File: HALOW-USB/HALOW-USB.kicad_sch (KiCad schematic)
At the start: 12 parts, among them U1 TLV75533PDBVR, U2 GT-USB-7010ASV

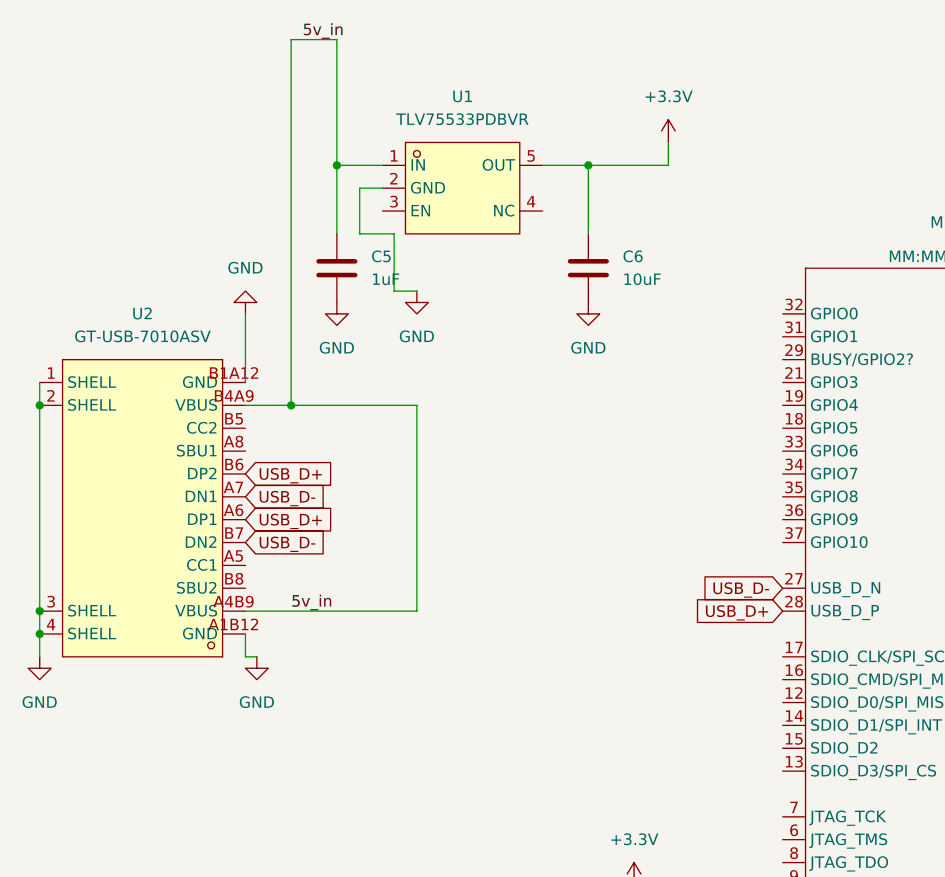
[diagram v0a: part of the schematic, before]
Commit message: trace work
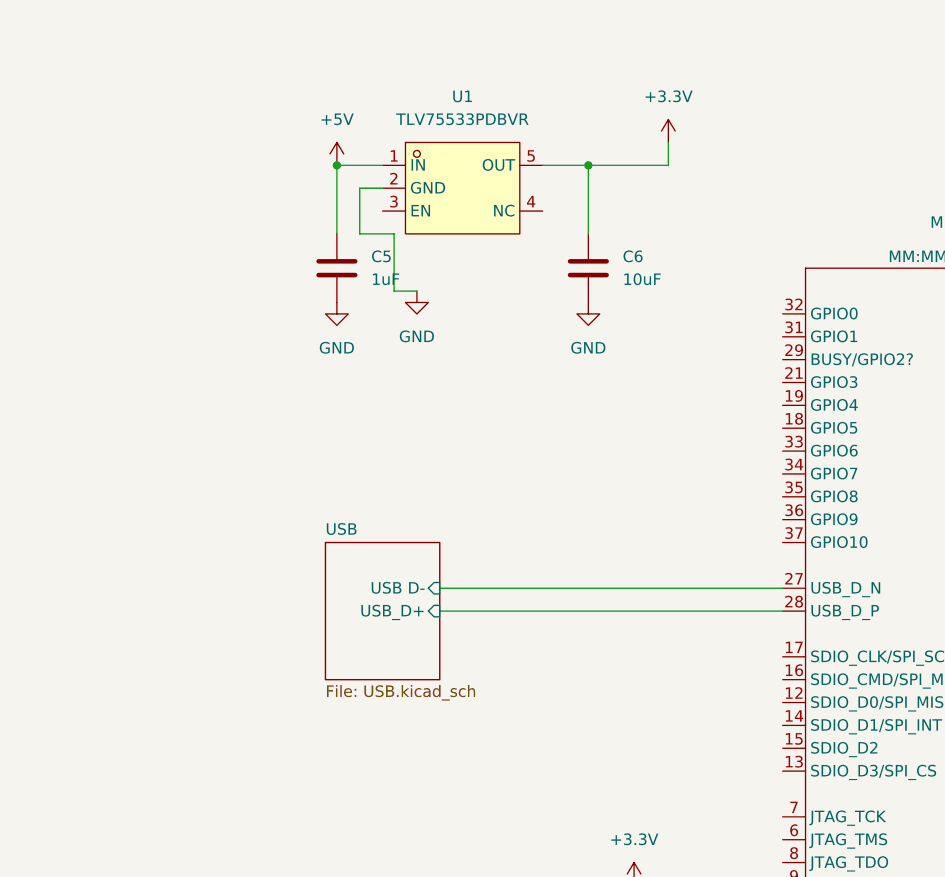
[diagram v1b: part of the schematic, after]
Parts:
- removed U2: GT-USB-7010ASV, easyeda2kicad:USB-C-SMD_G-SWITCH_GT-USB-7010ASV, symbol easyeda2kicad:GT-USB-7010ASV
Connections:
- net 5v_in renamed +5V
- net USB_D+ renamed USB/USB_D+
- net USB_D- renamed USB/USB D-
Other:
- added sheet USB (USB.kicad_sch)
